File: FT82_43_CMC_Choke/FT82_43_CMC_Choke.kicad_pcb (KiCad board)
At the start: 2 copper layers, 80.2 x 26.1 mm, 16 parts, among them J1 Conn_01x01_Pin, J4 Conn_01x01_Pin, J6 Conn_01x01_Pin

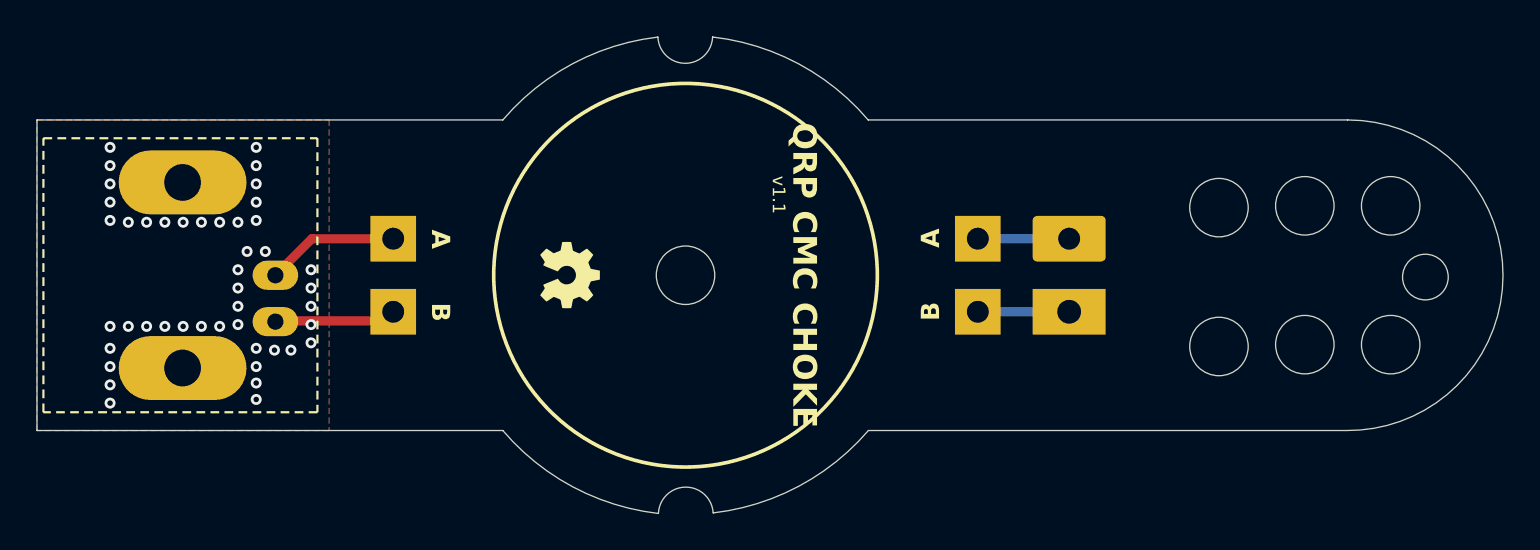
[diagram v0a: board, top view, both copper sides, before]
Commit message: PCB v1_1 :)
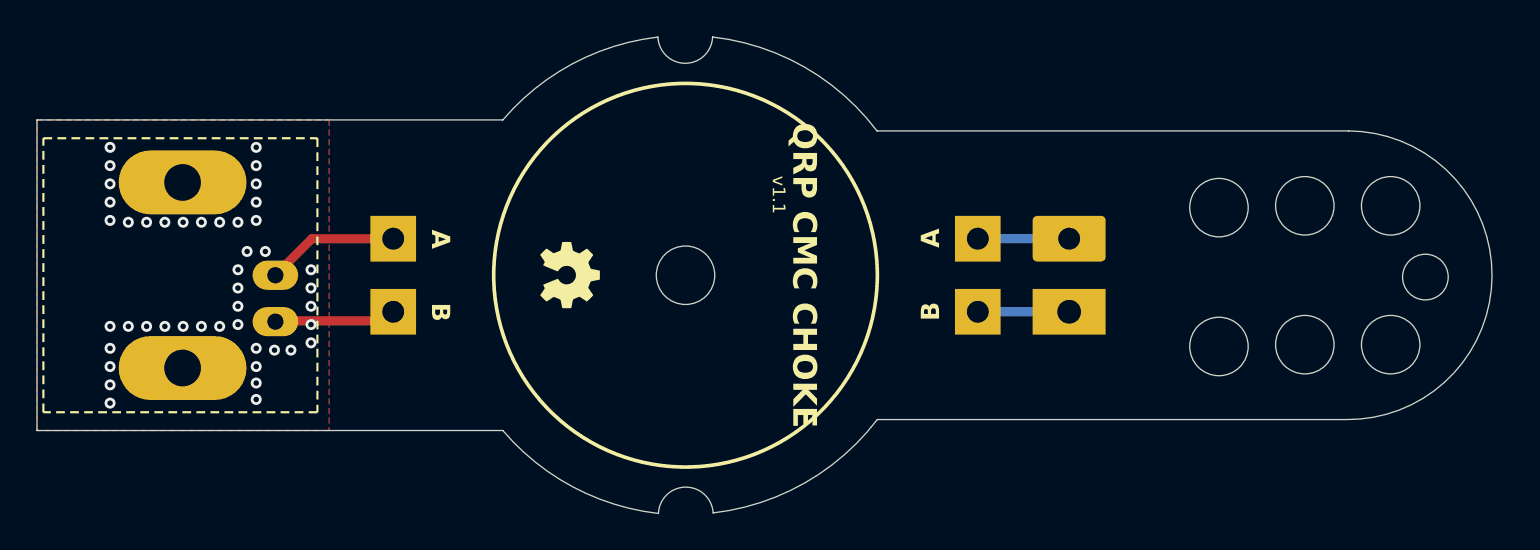
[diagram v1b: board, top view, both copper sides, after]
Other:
- board size 80.2 x 26.1 mm -> 79.6 x 26.1 mm
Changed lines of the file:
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@@
 	)
 	(gr_arc
-		(start 186.448305 91.699835)
-		(mid 194.948429 100.226401)
-		(end 186.395504 108.700001)
+		(start 186.491479 92.29992)
+		(mid 194.348343 100.249509)
+		(end 186.392462 108.100001)
 		(stroke
 			(width 0.05)
@@
 	)
 	(gr_arc
-		(start 160.210574 108.699999)
-		(mid 156.387693 111.756931)
-		(end 151.713625 113.210321)
+		(start 160.696265 108.099999)
+		(mid 156.725965 111.570978)
+		(end 151.713626 113.21032)
 		(stroke
 			(width 0.05)
@@
 	(gr_arc
 		(start 151.68258 87.159712)
-		(mid 156.373844 88.618514)
-		(end 160.2 91.700168)
+		(mid 156.710296 88.804246)
+		(end 160.680381 92.300079)
 		(stroke
 			(width 0.05)
@@
 	)
 	(gr_line
-		(start 186.395498 108.700001)
-		(end 160.210574 108.699999)
+		(start 186.392509 108.100001)
+		(end 160.696265 108.099999)
 		(stroke
 			(width 0.05)
@@
 	)
 	(gr_line
-		(start 186.448305 91.699835)
-		(end 160.2 91.7)
+		(start 186.491479 92.29992)
+		(end 160.680381 92.300079)
 		(stroke
 			(width 0.05)
